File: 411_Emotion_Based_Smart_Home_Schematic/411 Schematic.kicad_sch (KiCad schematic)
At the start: 9 parts, among them Q1 NSS1C301ET4G, Q2 NSS1C301ET4G, Q3 NSS1C301ET4G, U4 HC-SR04

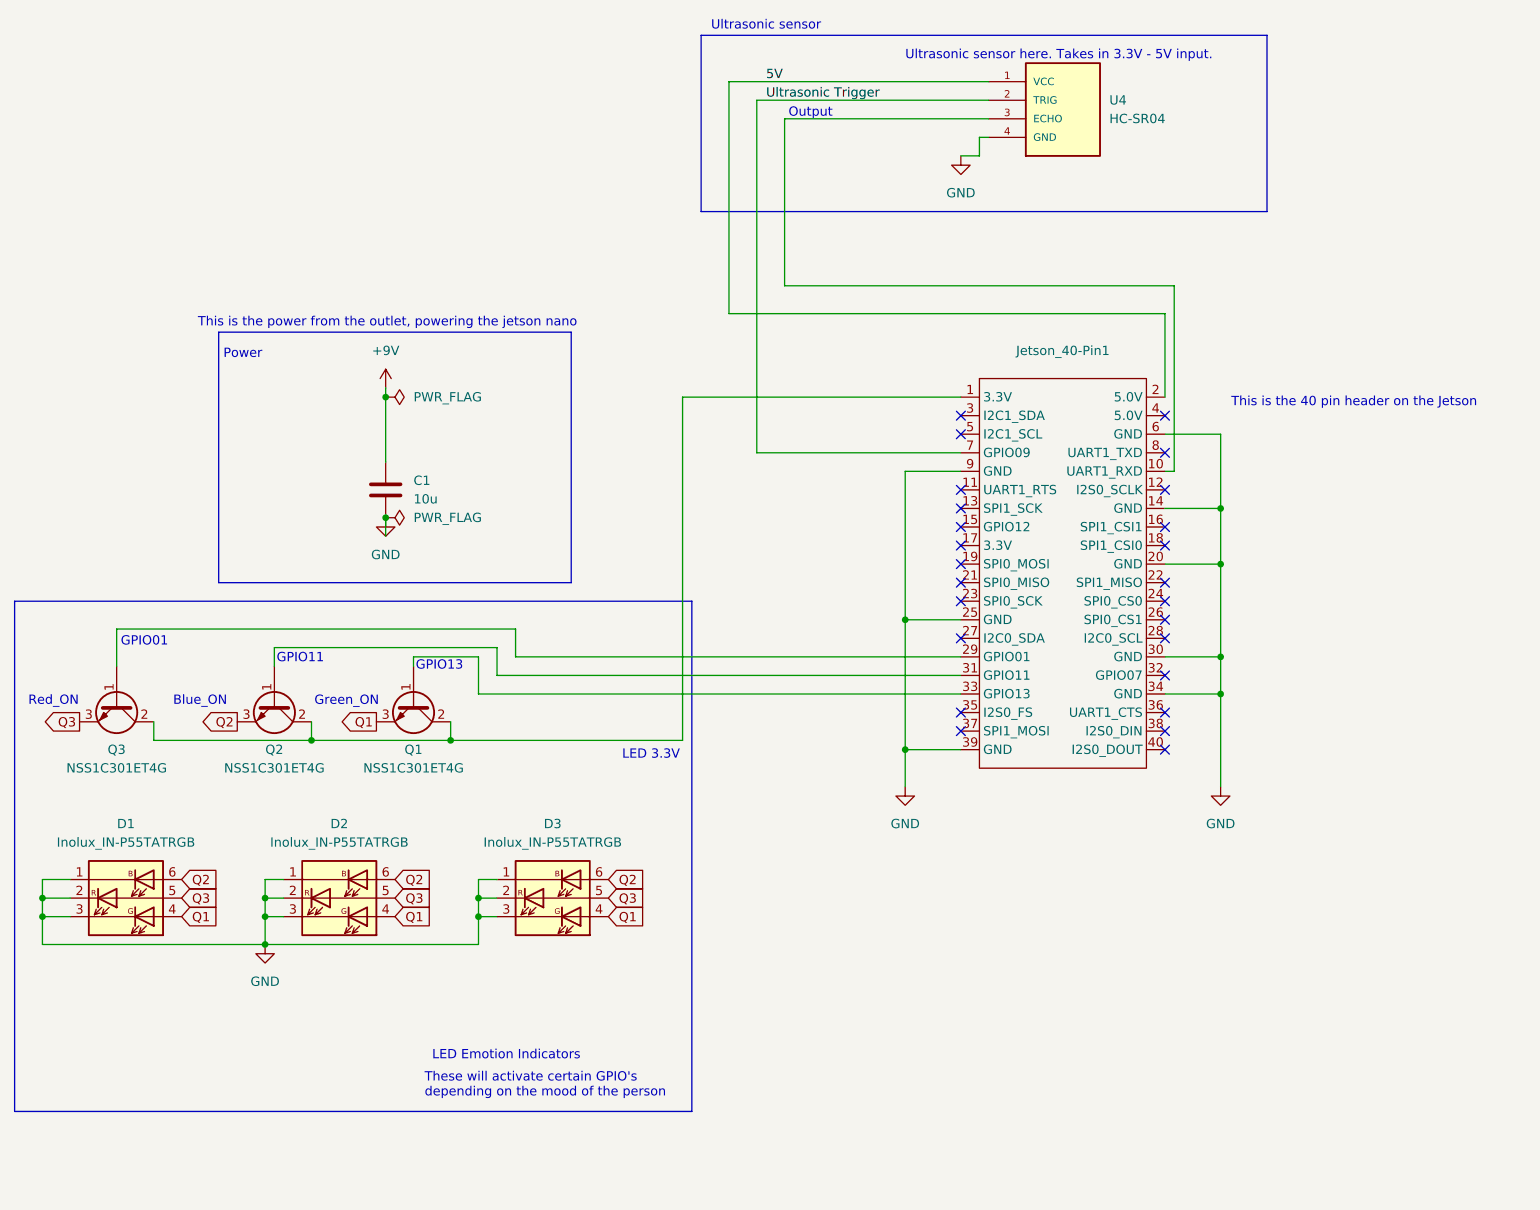
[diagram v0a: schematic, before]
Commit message: Updated schematic.
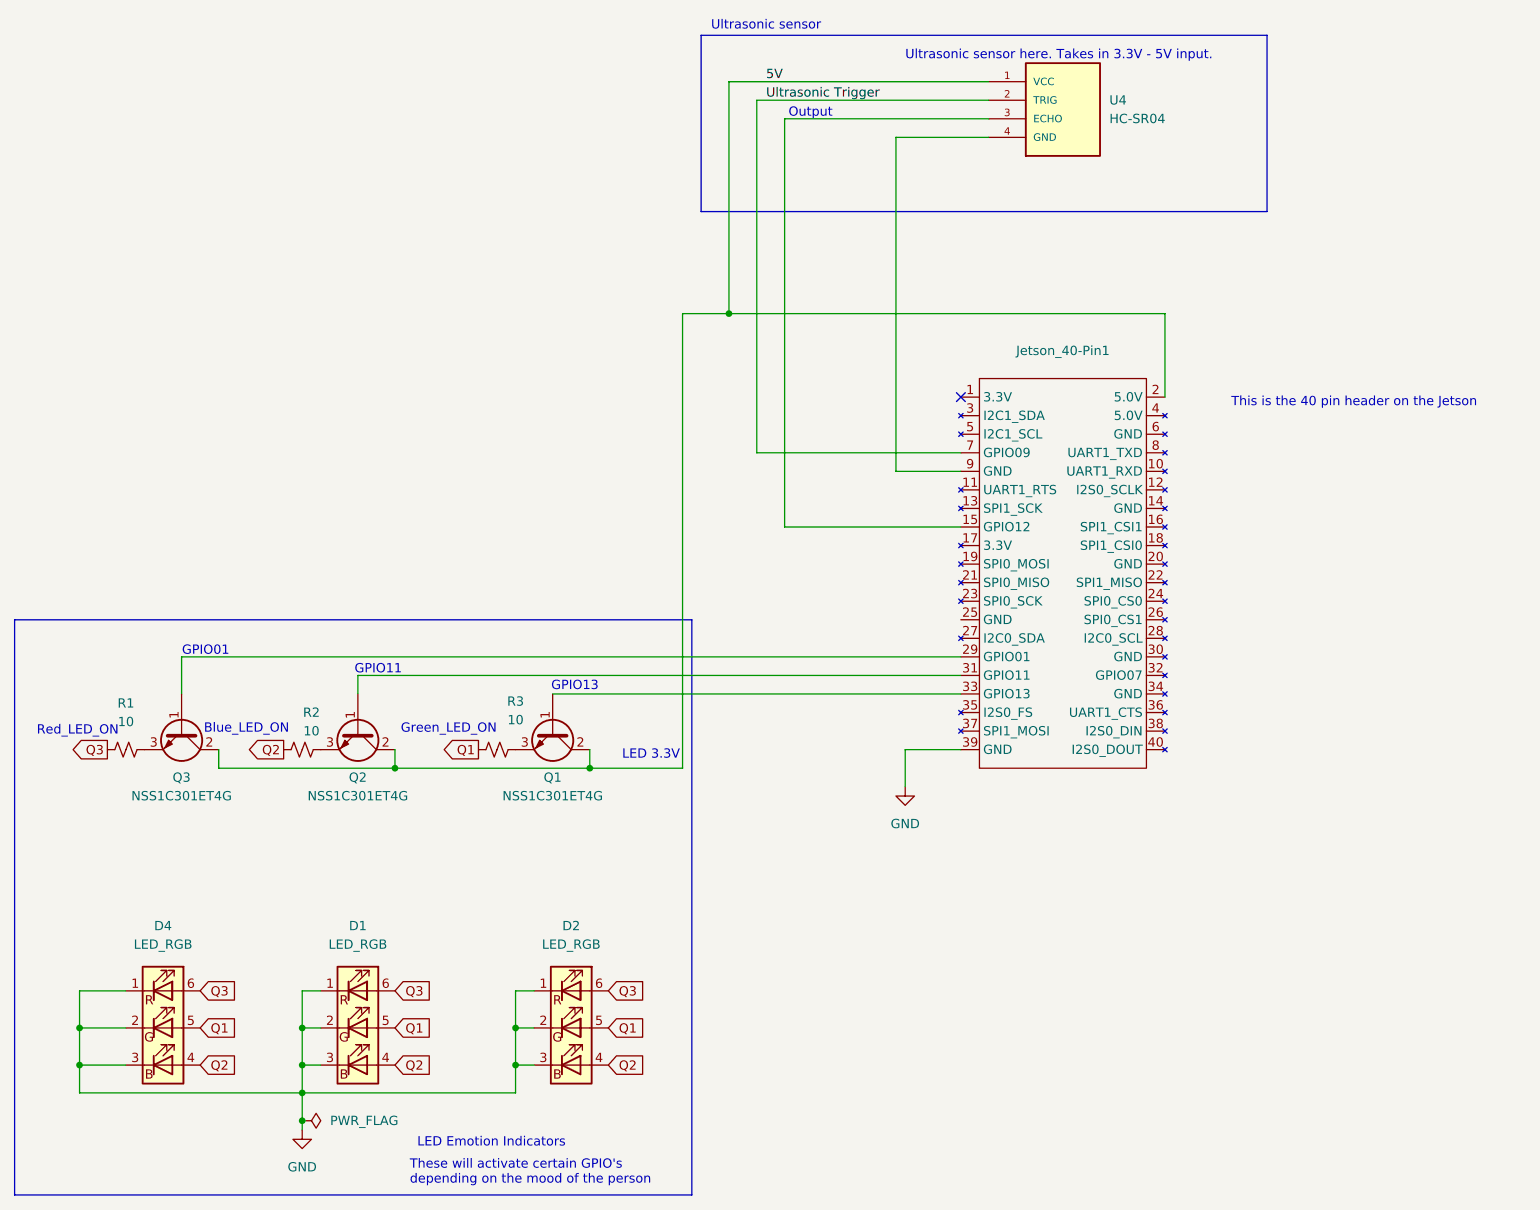
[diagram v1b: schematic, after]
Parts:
- removed C1: 10u, symbol Device:C
- removed D1, D2, D3: Inolux_IN-P55TATRGB, LED_SMD:LED_Inolux_IN-P55TATRGB_PLCC6_5.0x5.5mm_P1.8mm, symbol LED:Inolux_IN-P55TATRGB
- added D1, D2, D4: LED_RGB, LED_SMD:LED_RGB_5050-6, symbol Device:LED_RGB
- added R1, R2, R3: 10, Resistor_THT:R_Axial_DIN0411_L9.9mm_D3.6mm_P5.08mm_Vertical, symbol Device:R_Small_US
- Q1, Q2, Q3: footprint Transistor411Library:DPAK-4_6P22X6P73_ONS -> NSS1C301ET4G:DPAK-4_6P22X6P73_ONS
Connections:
- net 5V: now also Q1.2 (C), Q2.2 (C), Q3.2 (C)
- net GND: now also D1.1 (RK), D1.2 (GK), D1.3 (BK), D2.1 (RK), D2.2 (GK), D2.3 (BK), D4.1 (RK), D4.2 (GK), D4.3 (BK); no longer Jetson_40-Pin1.14 (GND), Jetson_40-Pin1.20 (GND), Jetson_40-Pin1.25 (GND), Jetson_40-Pin1.30 (GND), Jetson_40-Pin1.34 (GND), Jetson_40-Pin1.6 (GND), Jetson_40-Pin1.9 (GND), U4.4 (GND)
- net Q1: now also D1.5 (GA), D2.5 (GA), D4.5 (GA), R3.1; no longer Q1.3 (E)
- net Q2: now also D1.4 (BA), D2.4 (BA), D4.4 (BA), R2.1; no longer Q2.3 (E)
- net Q3: now also D1.6 (RA), D2.6 (RA), D4.6 (RA), R1.1; no longer Q3.3 (E)
- net at Jetson_40-Pin1.10 (UART1_RXD): no longer U4.3 (ECHO)
- net at Jetson_40-Pin1.15 (GPIO12): now also U4.3 (ECHO)
- new net: Jetson_40-Pin1.9 (GND), U4.4 (GND)
- new net: Q2.3 (E), R2.2
- new net: Q3.3 (E), R1.2
- new net: Q1.3 (E), R3.2
- now unconnected: Jetson_40-Pin1.1 (3.3V)
- no-connect marks 25 -> 1
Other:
- note added: "Blue_LED_ON"
- note added: "Green_LED_ON"
- note added: "Red_LED_ON"
- note removed: "Blue_ON"
- note removed: "Green_ON"
- note removed: "Power"
- note removed: "Red_ON"
- note removed: "This is the power from the outlet, powering the jetson nano"
- moved on the sheet: Q1, Q2, Q3
